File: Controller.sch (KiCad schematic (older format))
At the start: 21 parts, among them J1 ToArduino, J2 FromArduino, J3 Power12V, J4 A0 Sensor, J5 D12, J6 D4 - Heat, J7 D11, J8 D5-Fan, Q1 IRF-Heat, Q2 IRF-Fan, SW1 Button +, SW2 Button -

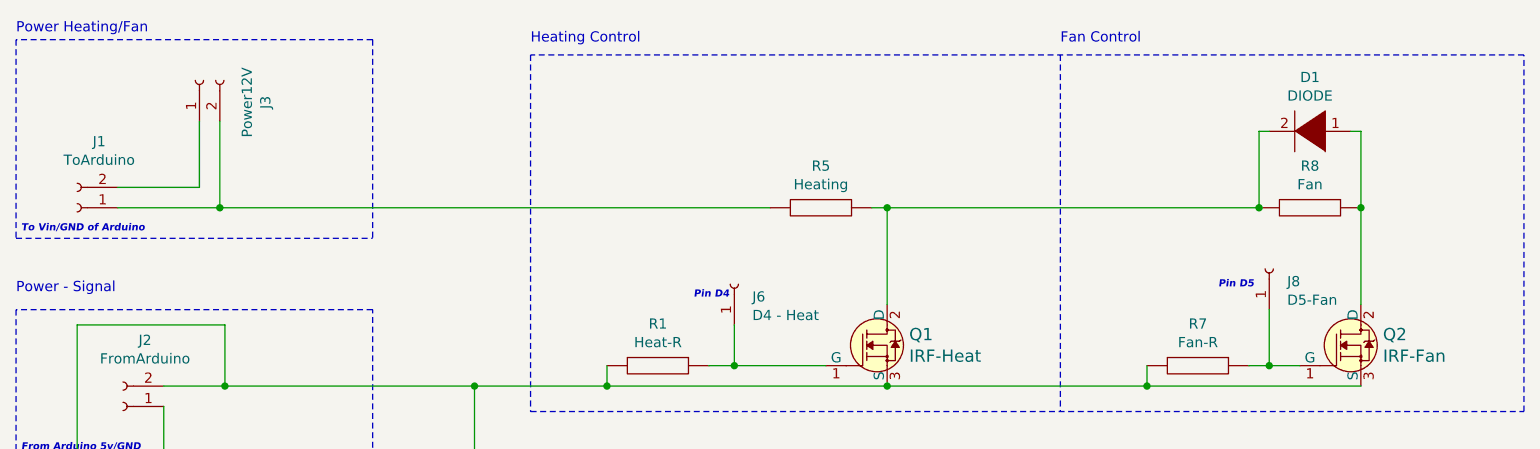
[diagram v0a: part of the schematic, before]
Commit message: version 1.1 #4 #5
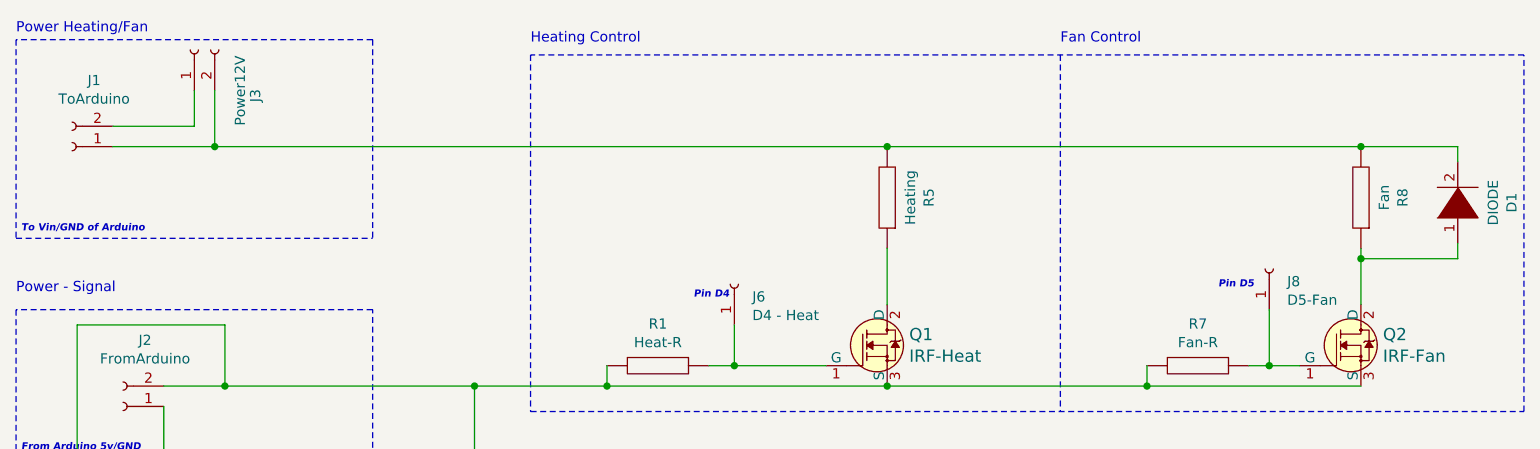
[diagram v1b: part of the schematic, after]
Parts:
- D1: footprint Diode_THT:D_DO-15_P15.24mm_Horizontal -> Diode_THT:D_DO-15_P5.08mm_Vertical_KathodeUp
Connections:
- net at Q1.2 (D), R5.1: no longer D1.2 (A), R8.2
- net at J1.1 (Pin_1), J3.2 (Pin_2), R5.2: now also D1.2 (A), R8.2
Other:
- moved on the sheet: D1, J1, J3, R5, R8
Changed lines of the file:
@@
 L pspice:R R8
 U 1 1 60B01F9C
-P 6875 1425
-F 0 "R8" V 6670 1425 50  0000 C CNN
-F 1 "Fan" V 6761 1425 50  0000 C CNN
-F 2 "Connector_PinSocket_2.54mm:PinSocket_1x02_P2.54mm_Vertical" H 6875 1425 50  0001 C CNN
-F 3 "~" H 6875 1425 50  0001 C CNN
-	1    6875 1425
-	0    1    1    0
+P 7125 1375
+F 0 "R8" V 6920 1375 50  0000 C CNN
+F 1 "Fan" V 7011 1375 50  0000 C CNN
+F 2 "Connector_PinSocket_2.54mm:PinSocket_1x02_P2.54mm_Vertical" H 7125 1375 50  0001 C CNN
+F 3 "~" H 7125 1375 50  0001 C CNN
+	1    7125 1375
+	-1   0    0    1
 $EndComp
 $Comp
 L pspice:R R5
 U 1 1 60B02699
-P 4475 1425
-F 0 "R5" V 4270 1425 50  0000 C CNN
-F 1 "Heating" V 4361 1425 50  0000 C CNN
-F 2 "Connector_PinSocket_2.54mm:PinSocket_1x02_P2.54mm_Vertical" H 4475 1425 50  0001 C CNN
-F 3 "~" H 4475 1425 50  0001 C CNN
-	1    4475 1425
-	0    1    1    0
+P 4800 1375
+F 0 "R5" V 4595 1375 50  0000 C CNN
+F 1 "Heating" V 4686 1375 50  0000 C CNN
+F 2 "Connector_PinSocket_2.54mm:PinSocket_1x02_P2.54mm_Vertical" H 4800 1375 50  0001 C CNN
+F 3 "~" H 4800 1375 50  0001 C CNN
+	1    4800 1375
+	-1   0    0    1
 $EndComp
 $Comp
 L Connector:Conn_01x02_Female J1
 U 1 1 60B02D22
-P 825 1425
-F 0 "J1" H 717 1100 50  0000 C CNN
-F 1 "ToArduino" H 717 1191 50  0000 C CNN
-F 2 "Connector_PinSocket_2.54mm:PinSocket_1x02_P2.54mm_Vertical" H 825 1425 50  0001 C CNN
-F 3 "~" H 825 1425 50  0001 C CNN
-	1    825  1425
+P 800 1125
+F 0 "J1" H 692 800 50  0000 C CNN
+F 1 "ToArduino" H 692 891 50  0000 C CNN
+F 2 "Connector_PinSocket_2.54mm:PinSocket_1x02_P2.54mm_Vertical" H 800 1125 50  0001 C CNN
+F 3 "~" H 800 1125 50  0001 C CNN
+	1    800  1125
 	-1   0    0    1
 $EndComp
@@
 L pspice:DIODE D1
 U 1 1 60B0CC70
-P 6875 1050
-F 0 "D1" H 6875 785 50  0000 C CNN
-F 1 "DIODE" H 6875 876 50  0000 C CNN
-F 2 "Diode_THT:D_DO-15_P15.24mm_Horizontal" H 6875 1050 50  0001 C CNN
-F 3 "~" H 6875 1050 50  0001 C CNN
-	1    6875 1050
-	-1   0    0    1
+P 7600 1400
+F 0 "D1" H 7600 1135 50  0000 C CNN
+F 1 "DIODE" H 7600 1226 50  0000 C CNN
+F 2 "Diode_THT:D_DO-15_P5.08mm_Vertical_KathodeUp" H 7600 1400 50  0001 C CNN
+F 3 "~" H 7600 1400 50  0001 C CNN
+	1    7600 1400
+	0    -1   -1   0
 $EndComp
 Wire Notes Line
@@
 Wire Wire Line
 	6675 2200 6825 2200
-Wire Wire Line
-	7125 1425 7125 1900
-Wire Wire Line
-	7075 1050 7125 1050
-Wire Wire Line
-	7125 1050 7125 1425
-Connection ~ 7125 1425
-Wire Wire Line
-	6675 1050 6625 1050
-Wire Wire Line
-	6625 1050 6625 1425
-Connection ~ 6625 1425
 $Comp
 L Switch:SW_Push_Dual SW1
@@
 Wire Wire Line
 	4800 5075 4325 5075
-Wire Wire Line
-	4725 1425 4800 1425
-Wire Wire Line
-	4800 1900 4800 1425
-Connection ~ 4800 1425
-Wire Wire Line
-	4800 1425 6625 1425
 Text Notes 550  1550 0    35   Italic 7
 To Vin/GND of Arduino
@@
 	2275 600  2275 1575
 Wire Wire Line
-	1425 1325 1025 1325
+	1400 1025 1000 1025
 $Comp
 L Connector:Conn_01x02_Female J3
 U 1 1 60B67757
-P 1425 800
-F 0 "J3" H 1317 475 50  0000 C CNN
-F 1 "Power12V" H 1317 566 50  0000 C CNN
-F 2 "Connector_BarrelJack:BarrelJack_CUI_PJ-063AH_Horizontal" H 1425 800 50  0001 C CNN
-F 3 "~" H 1425 800 50  0001 C CNN
-	1    1425 800
+P 1400 650
+F 0 "J3" H 1175 350 50  0000 C CNN
+F 1 "Power12V" H 1200 425 50  0000 C CNN
+F 2 "Connector_BarrelJack:BarrelJack_CUI_PJ-063AH_Horizontal" H 1400 650 50  0001 C CNN
+F 3 "~" H 1400 650 50  0001 C CNN
+	1    1400 650
 	0    -1   -1   0
 $EndComp
 Wire Wire Line
-	1425 1000 1425 1325
+	1400 850  1400 1025
 Wire Wire Line
 	6050 4550 6050 4375
@@
 	1550 2300 2775 2300
 Wire Wire Line
-	1025 1425 1525 1425
-Wire Wire Line
-	1525 1000 1525 1425
-Connection ~ 1525 1425
-Wire Wire Line
-	1525 1425 4225 1425
+	1000 1125 1500 1125
 $Comp
 L pspice:R R6
@@
 	-1   0    0    1
 $EndComp
+Wire Wire Line
+	1500 850  1500 1125
+Wire Wire Line
+	4800 1125 1500 1125
+Connection ~ 1500 1125
+Wire Wire Line
+	4800 1625 4800 1900
+Wire Wire Line
+	4800 1125 7125 1125
+Connection ~ 4800 1125
+Wire Wire Line
+	7125 1625 7125 1675
+Wire Wire Line
+	7600 1200 7600 1125
+Wire Wire Line
+	7600 1125 7125 1125
+Connection ~ 7125 1125
+Wire Wire Line
+	7600 1600 7600 1675
+Wire Wire Line
+	7600 1675 7125 1675
+Connection ~ 7125 1675
+Wire Wire Line
+	7125 1675 7125 1900
 $EndSCHEMATC
